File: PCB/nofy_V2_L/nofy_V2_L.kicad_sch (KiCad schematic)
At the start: 153 parts, among them J18 PIn1x4, J21 PIn1x4, J32 PIn1x4, J33 PIn1x4, SW1 SW_SPDT, SW10 SW_PUSH, SW11 SW_PUSH, SW12 SW_PUSH, SW13 SW_PUSH, SW14 SW_PUSH, SW15 SW_PUSH, SW16 SW_PUSH, SW17 SW_PUSH, SW18 SW_PUSH, SW19 SW_PUSH, SW2 SW_SPDT, SW20 SW_PUSH, SW21 SW_PUSH, SW22 SW_PUSH, SW23 SW_PUSH, SW24 SW_PUSH, SW25 SW_PUSH, SW26 SW_PUSH, SW27 SW_PUSH, SW28 SW_PUSH, SW29 SW_PUSH, SW3 RotaryEncoder, SW30 SW_PUSH, SW31 SW_PUSH, SW32 SW_PUSH, SW33 SW_PUSH, SW34 SW_PUSH, SW35 SW_PUSH, SW36 SW_PUSH, SW37 SW_PUSH, SW38 SW_PUSH, SW39 SW_PUSH, SW4 RotaryEncoder, SW40 SW_PUSH, SW41 SW_PUSH, SW42 SW_PUSH, SW43 SW_PUSH, SW44 SW_PUSH, SW45 SW_PUSH, SW46 SW_PUSH, SW47 SW_PUSH, SW48 SW_PUSH, SW49 SW_PUSH, SW5 SW_PUSH, SW50 SW_PUSH, SW51 SW_PUSH, SW52 SW_PUSH, SW53 SW_PUSH, SW54 SW_PUSH, SW55 SW_PUSH, SW6 SW_PUSH, SW7 SW_PUSH, SW8 SW_PUSH, SW9 SW_PUSH

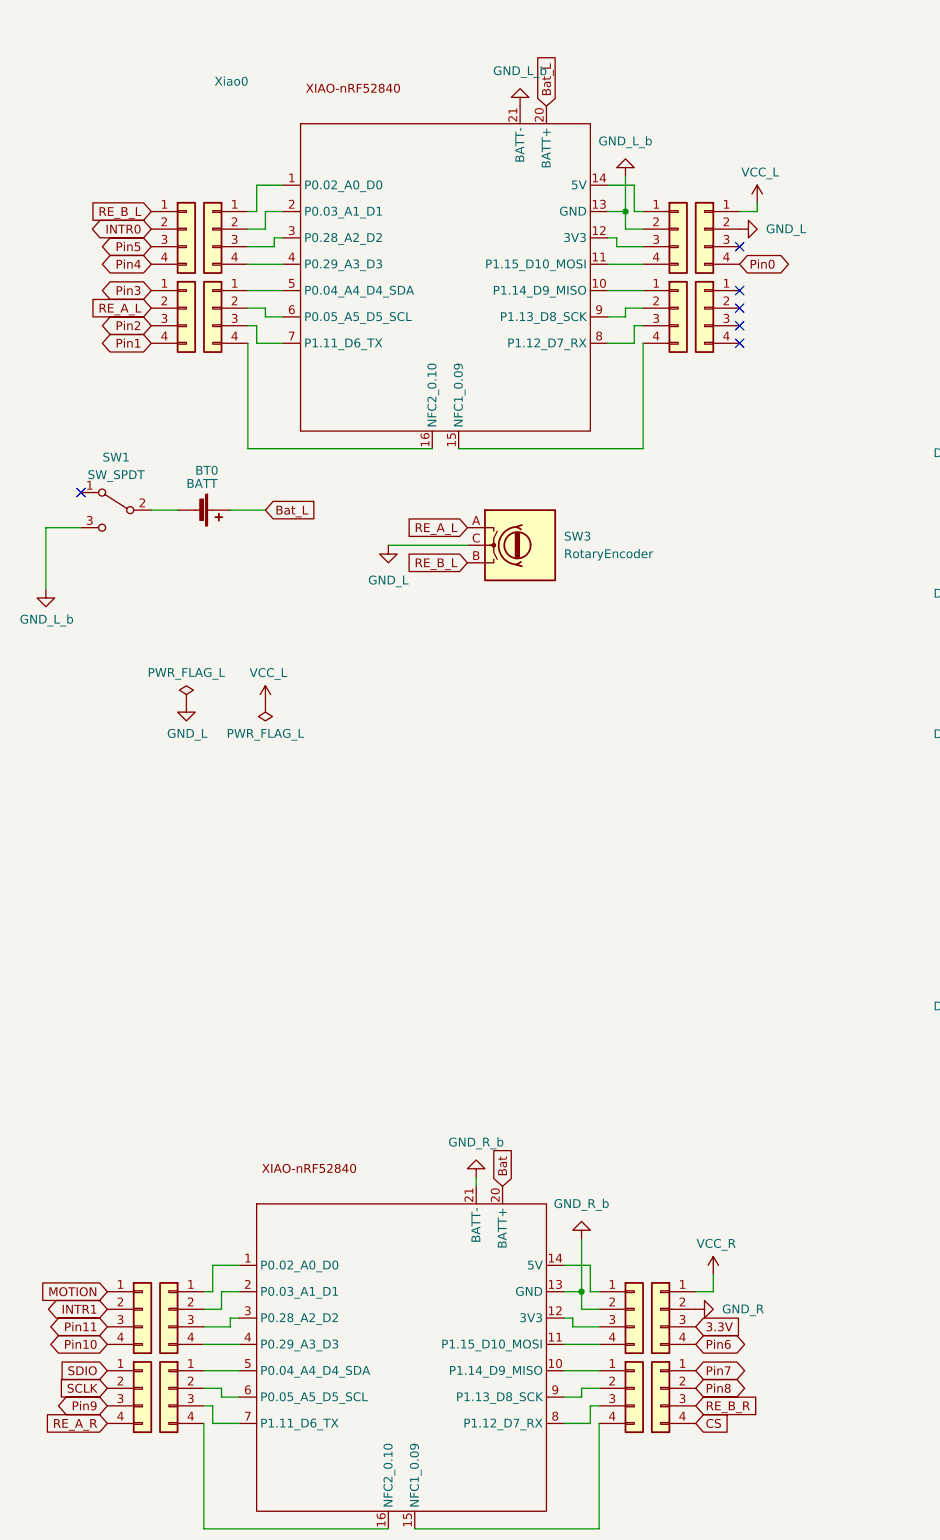
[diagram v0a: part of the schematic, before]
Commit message: pcb
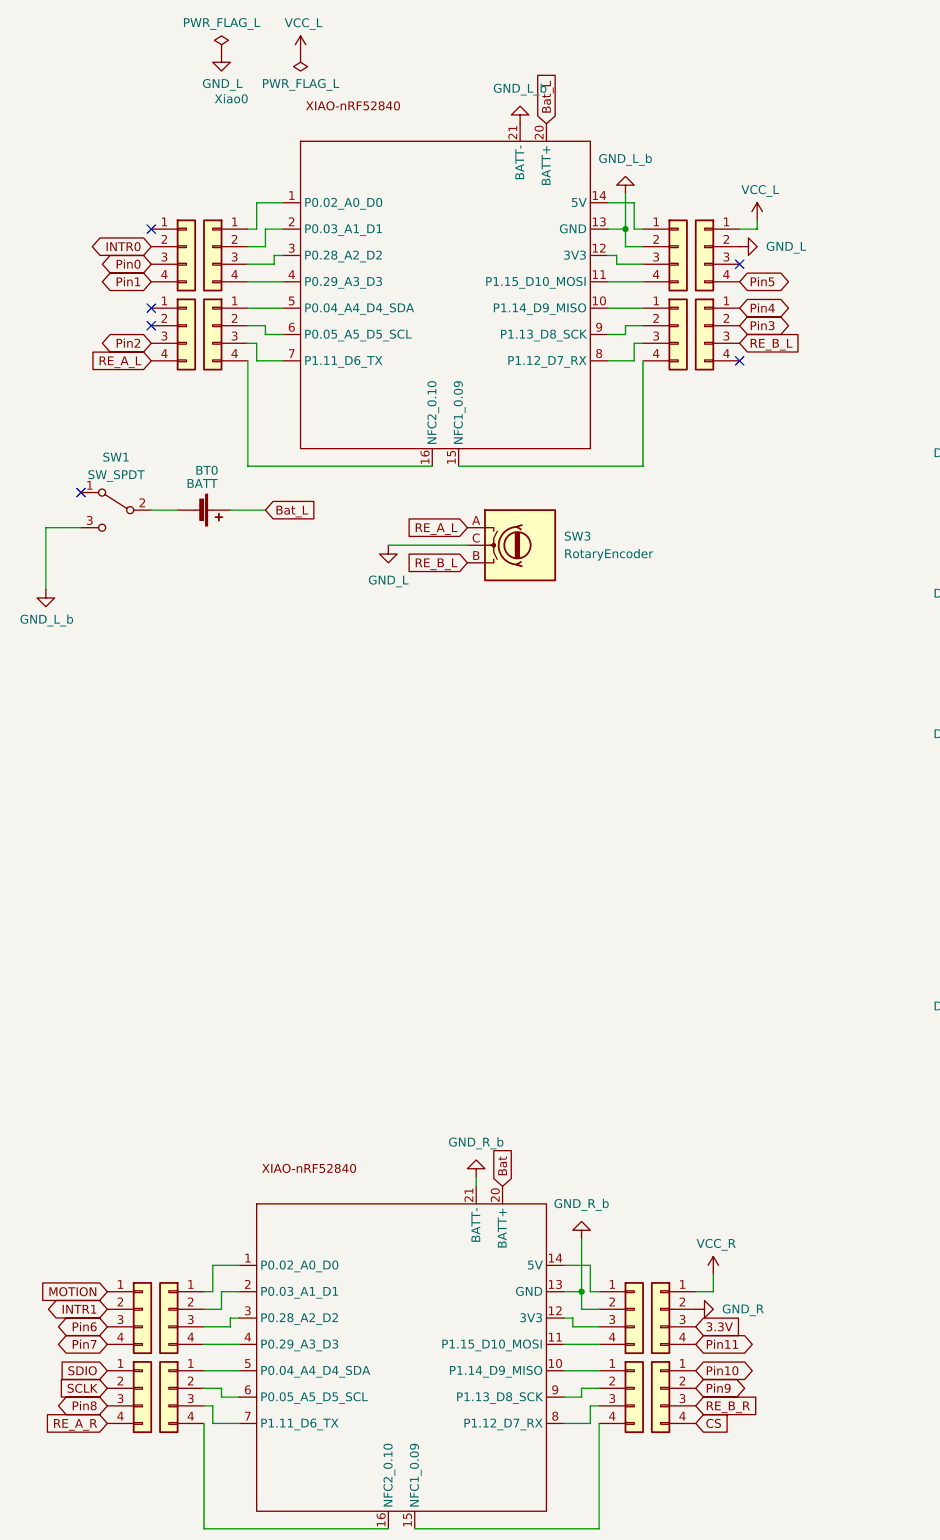
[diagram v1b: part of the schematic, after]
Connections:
- net Pin0: now also Con_L_0.3 (Pin_3); no longer Con_L_4.4 (Pin_4)
- net Pin1: now also Con_L_0.4 (Pin_4); no longer Con_L_2.4 (Pin_4)
- net Pin10: now also Con_L_14.1 (Pin_1); no longer Con_L_8.4 (Pin_4)
- net Pin11: now also Con_L_12.4 (Pin_4); no longer Con_L_8.3 (Pin_3)
- net Pin3: now also Con_L_6.2 (Pin_2); no longer Con_L_2.1 (Pin_1)
- net Pin4: now also Con_L_6.1 (Pin_1); no longer Con_L_0.4 (Pin_4)
- net Pin5: now also Con_L_4.4 (Pin_4); no longer Con_L_0.3 (Pin_3)
- net Pin6: now also Con_L_8.3 (Pin_3); no longer Con_L_12.4 (Pin_4)
- net Pin7: now also Con_L_8.4 (Pin_4); no longer Con_L_14.1 (Pin_1)
- net Pin8: now also Con_L_10.3 (Pin_3); no longer Con_L_14.2 (Pin_2)
- net Pin9: now also Con_L_14.2 (Pin_2); no longer Con_L_10.3 (Pin_3)
- net RE_A_L: now also Con_L_2.4 (Pin_4); no longer Con_L_2.2 (Pin_2)
- net RE_B_L: now also Con_L_6.3 (Pin_3); no longer Con_L_0.1 (Pin_1)
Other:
- moved on the sheet: Xiao0
